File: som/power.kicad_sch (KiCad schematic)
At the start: 1 part, among them U1 XC7A200T-3FBG484E

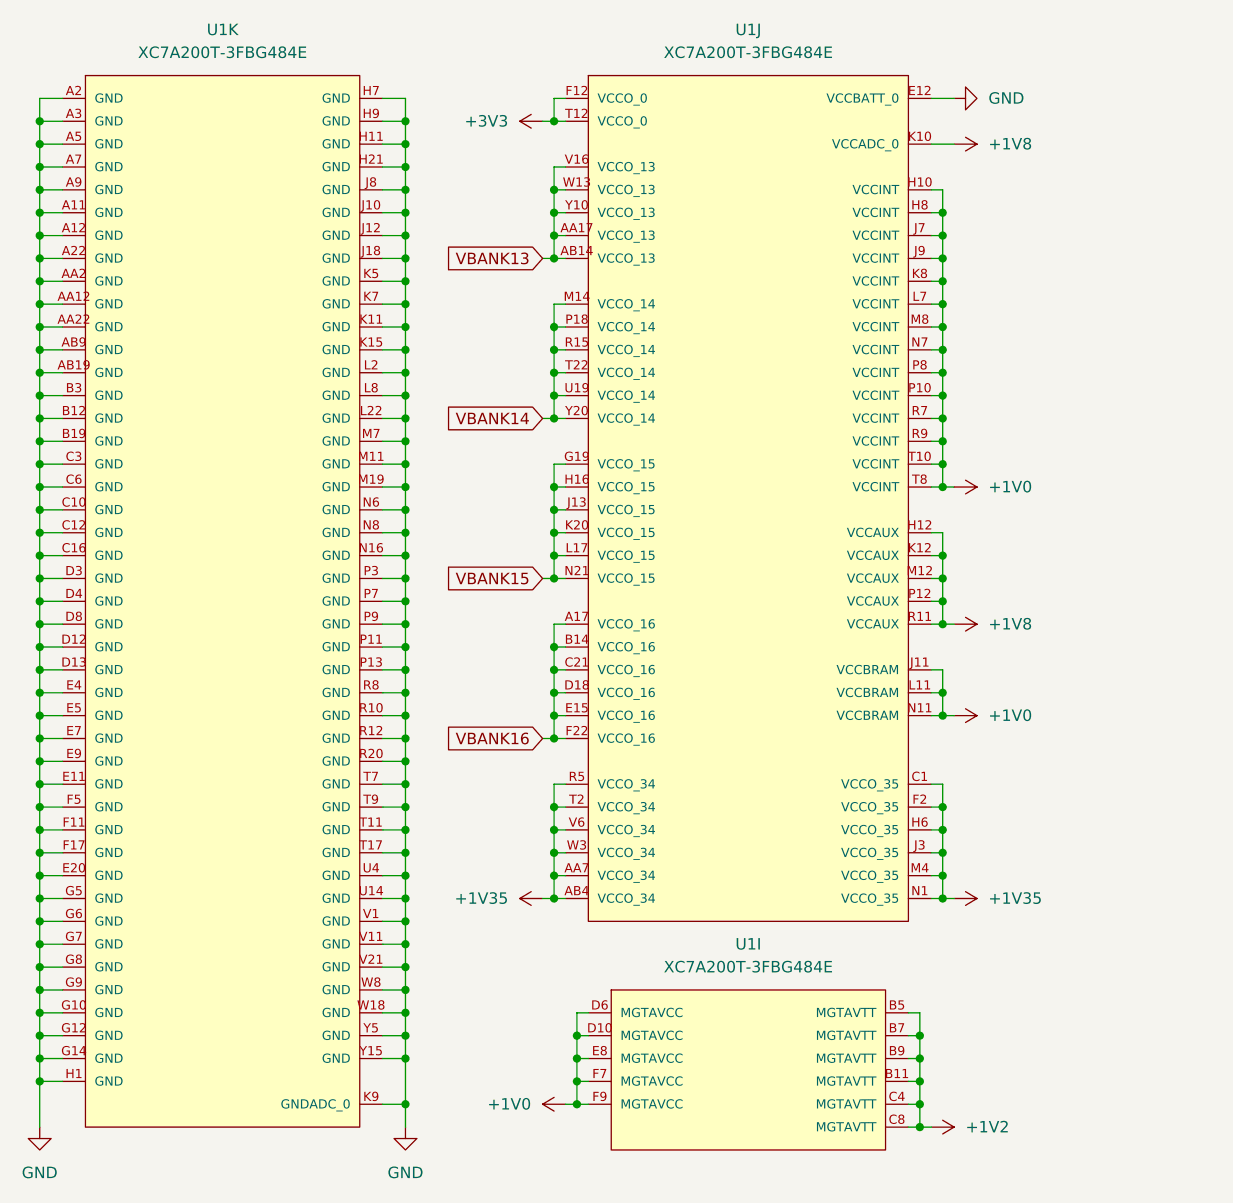
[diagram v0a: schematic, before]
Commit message: Mezz Power Tweak Ok
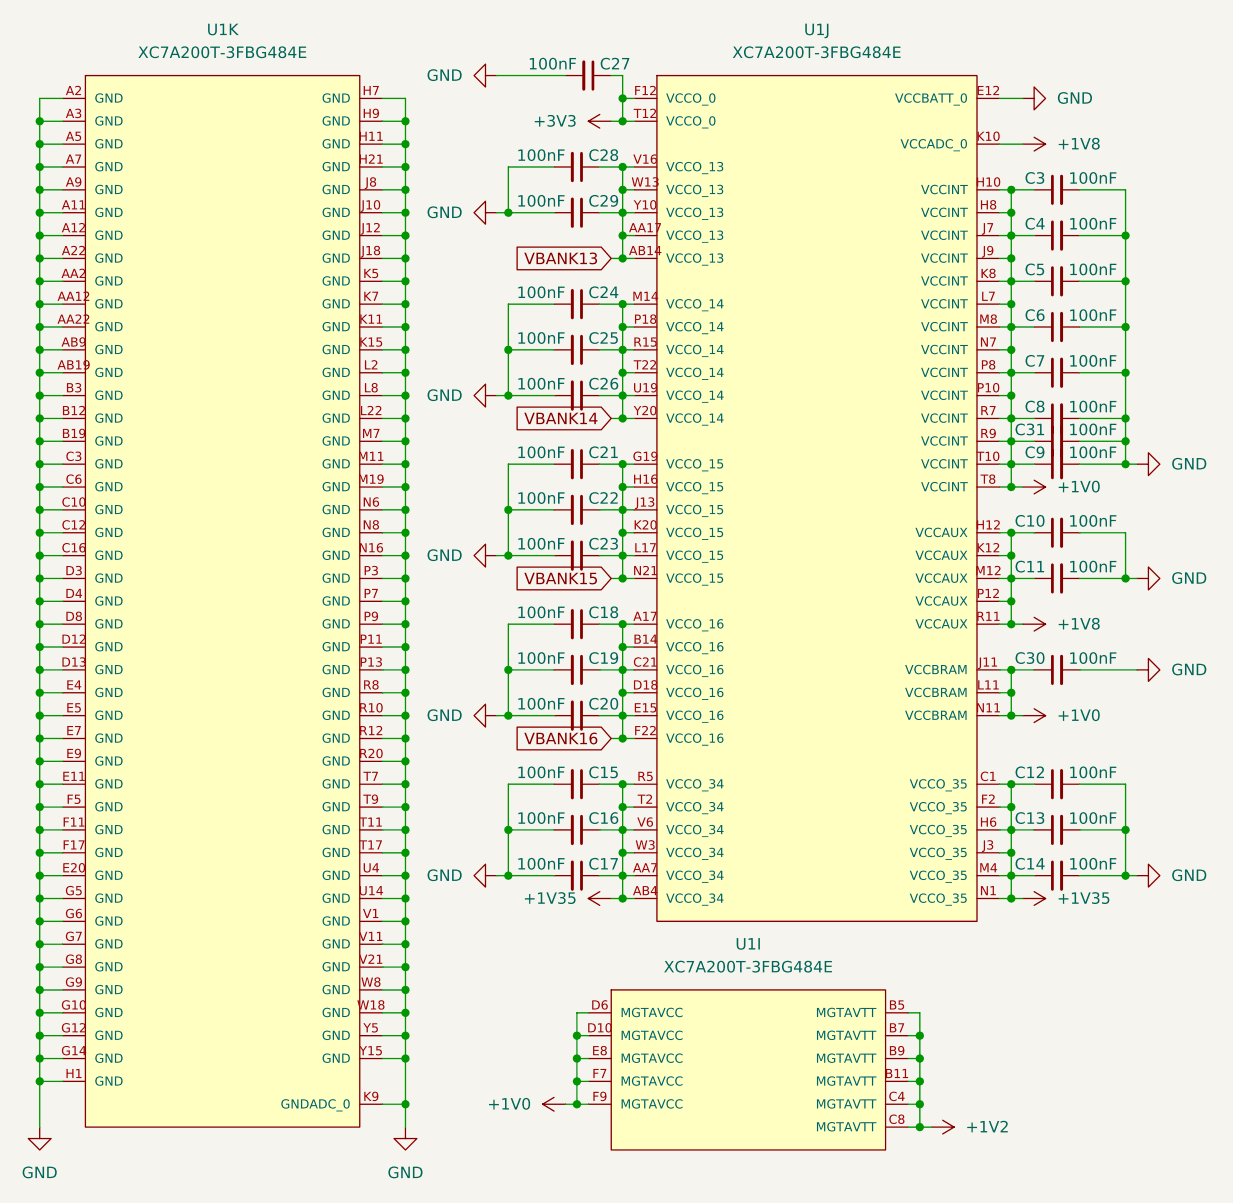
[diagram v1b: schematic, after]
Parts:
- added C10, C11, C12, C13, C14, C15, C16, C17, C18, C19, C20, C21, C22, C23, C24, C25, C26, C27, C28, C29, C3, C30, C31, C4, C5, C6, C7, C8, C9: 100nF, Capacitor_SMD:C_0402_1005Metric_Pad0.74x0.62mm_HandSolder, symbol Device:C_Small
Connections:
- net +1V0: now also C3.1, C30.1, C31.1, C4.1, C5.1, C6.1, C7.1, C8.1, C9.1
- net +1V35: now also C12.1, C13.1, C14.1, C15.1, C16.1, C17.1
- net +1V8: now also C10.1, C11.1
- net +3V3: now also C27.1
- net GND: now also C10.2, C11.2, C12.2, C13.2, C14.2, C15.2, C16.2, C17.2, C18.2, C19.2, C20.2, C21.2, C22.2, C23.2, C24.2, C25.2, C26.2, C27.2, C28.2, C29.2, C3.2, C30.2, C31.2, C4.2, C5.2, C6.2, C7.2, C8.2, C9.2
- net VBANK13: now also C28.1, C29.1
- net VBANK14: now also C24.1, C25.1, C26.1
- net VBANK15: now also C21.1, C22.1, C23.1
- net VBANK16: now also C18.1, C19.1, C20.1
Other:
- moved on the sheet: U1J
